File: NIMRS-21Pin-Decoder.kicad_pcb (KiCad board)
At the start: 4 copper layers, 30 x 23.5 mm, 90 parts, among them J1 21Pin Loco Socket, J2 U.FL, Q1 MMDT3904, Q2 MMDT3904, U1 ESP32-S3FN8, U2 MAX98357A, U4 DRV8213DSGR, U60 TPS63070, U70 TPS63070, X1 40Mhz

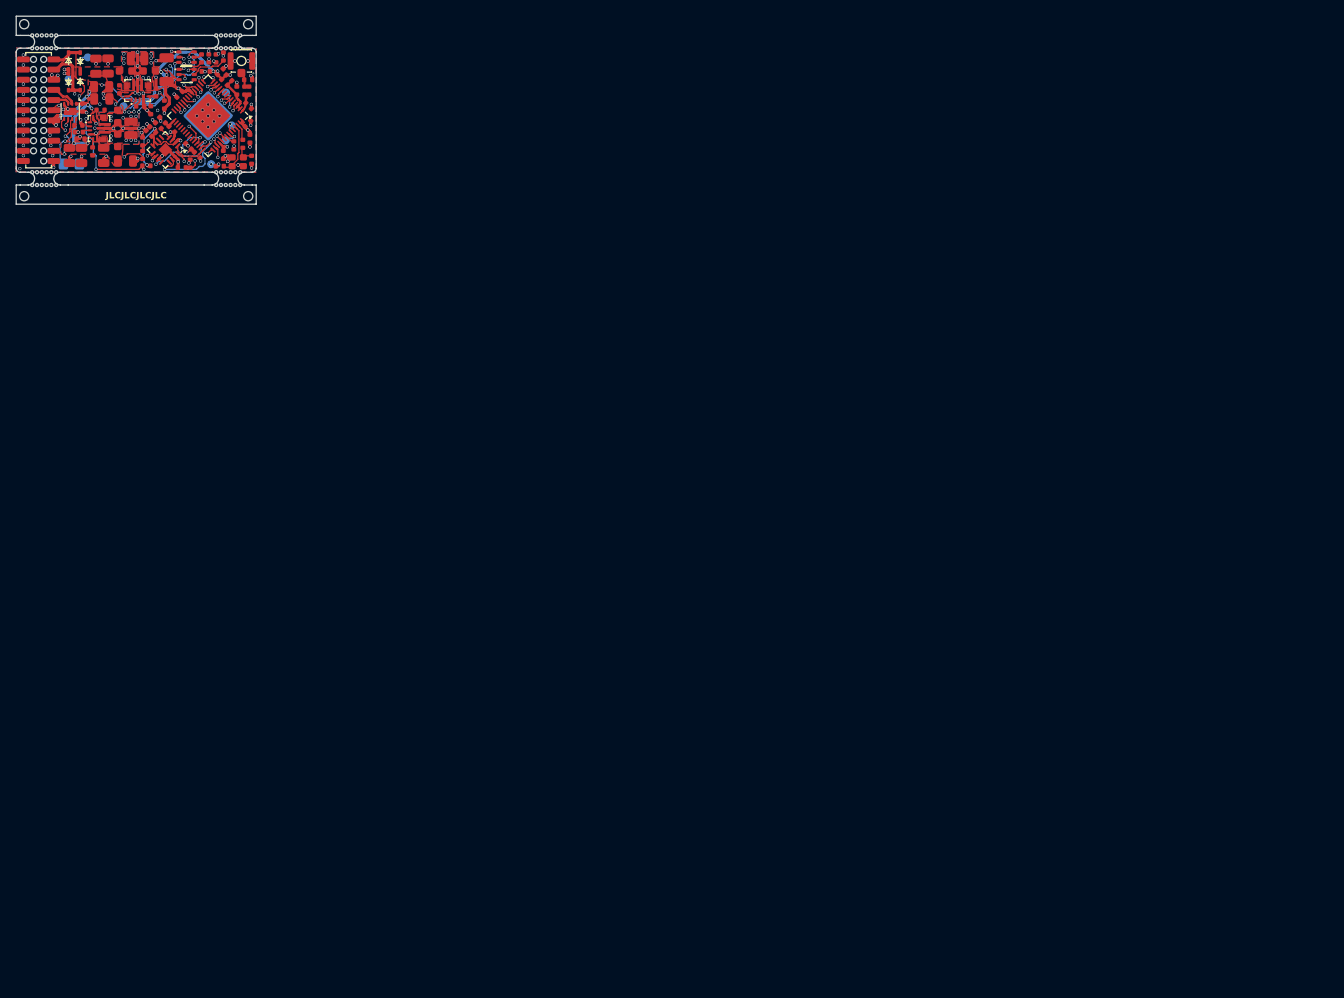
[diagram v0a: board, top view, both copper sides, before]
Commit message: Center PCB, Tidy up for r/PrintedCurcuitBoard
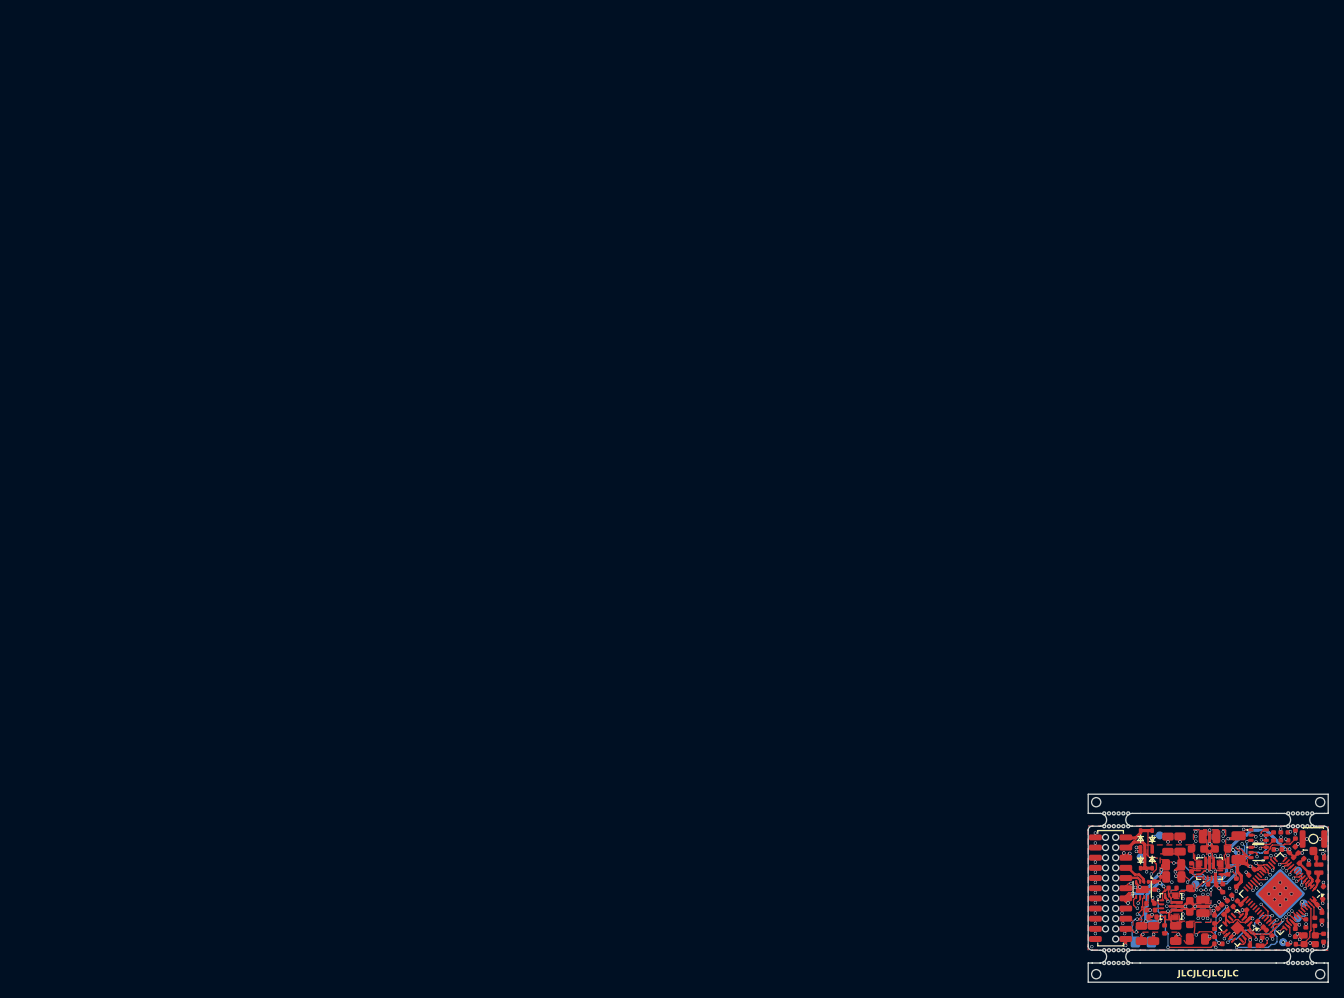
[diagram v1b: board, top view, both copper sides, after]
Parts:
- moved C1 165.6 mm to (161.6, 102.5)
- moved C10 165.6 mm to (159.4, 112.0)
- moved C11 165.6 mm to (154.4, 103.0)
- moved C12 165.6 mm to (163.1, 104.5)
- moved C13 165.6 mm to (163.0, 101.2)
- moved C15 165.6 mm to (151.1, 107.4)
- moved C16 165.6 mm to (150.6, 107.9)
- moved C17 165.6 mm to (142.3, 104.7)
- moved C2 165.6 mm to (159.5, 100.2)
- moved C4 165.6 mm to (157.7, 100.2)
- moved C5 165.6 mm to (163.2, 108.6)
- moved C6 165.6 mm to (152.3, 106.2)
- moved C60 165.6 mm to (144.7, 102.1)
- moved C61 165.6 mm to (144.7, 103.6)
- moved C62 165.6 mm to (146.7, 105.8)
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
